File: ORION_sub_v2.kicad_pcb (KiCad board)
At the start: 2 copper layers, 50 x 70 mm, 75 parts, among them J1 Conn_01x02, J10 Conn_01x01, J11 Conn_01x05, J12 Conn_01x03, J13 Conn_01x08, J2 Conn_01x03, J3 Conn_01x04, J4 Conn_01x02, J5 Conn_01x01, J6 Conn_01x04, J7 Conn_01x03, J8 Conn_01x04, J9 Conn_01x01, P1 CONN_01X06, Q1 BSS138, SW1 SW_Push, SW2 SW_Push, SW3 SW_Push, SW4 SW_Push, U1 STM32F303CBTx, U2 MAX3051, U3 AZ1117-3.3, U4 BD9G101G, X1 ceralock

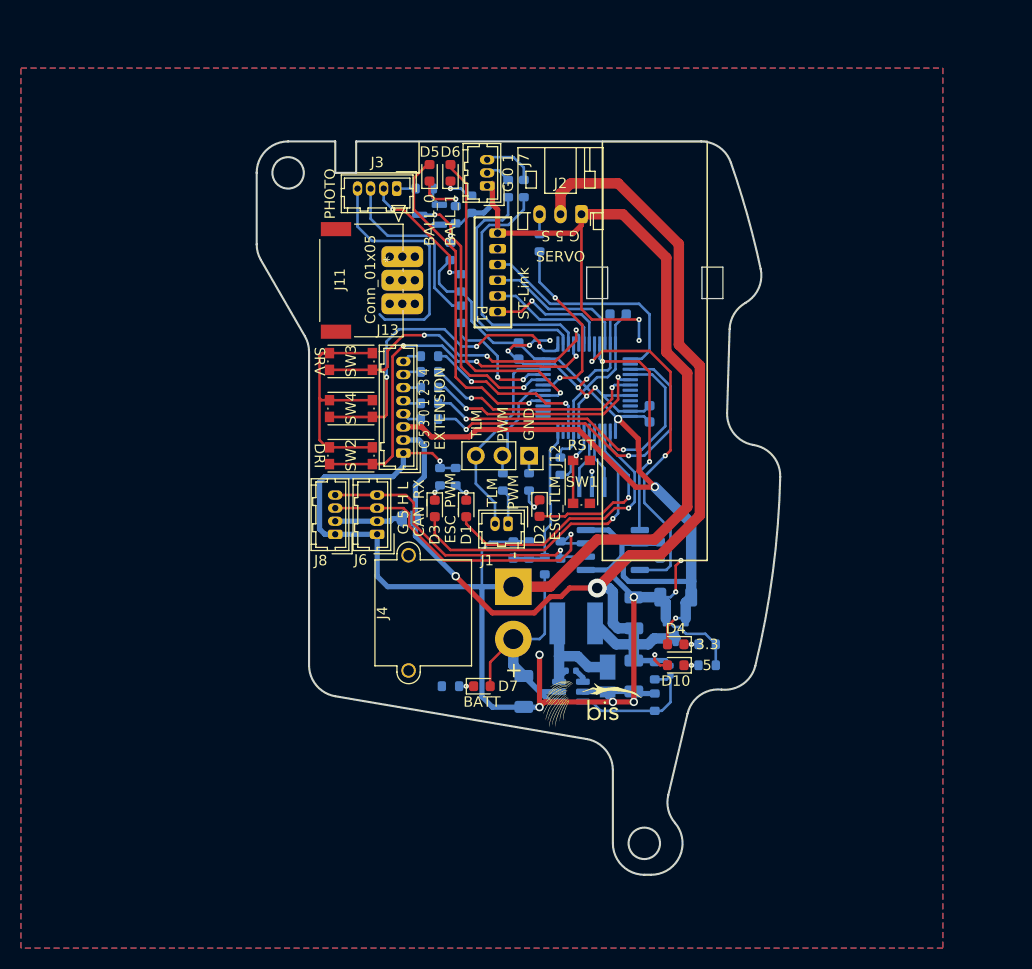
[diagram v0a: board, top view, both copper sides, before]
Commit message: 更新
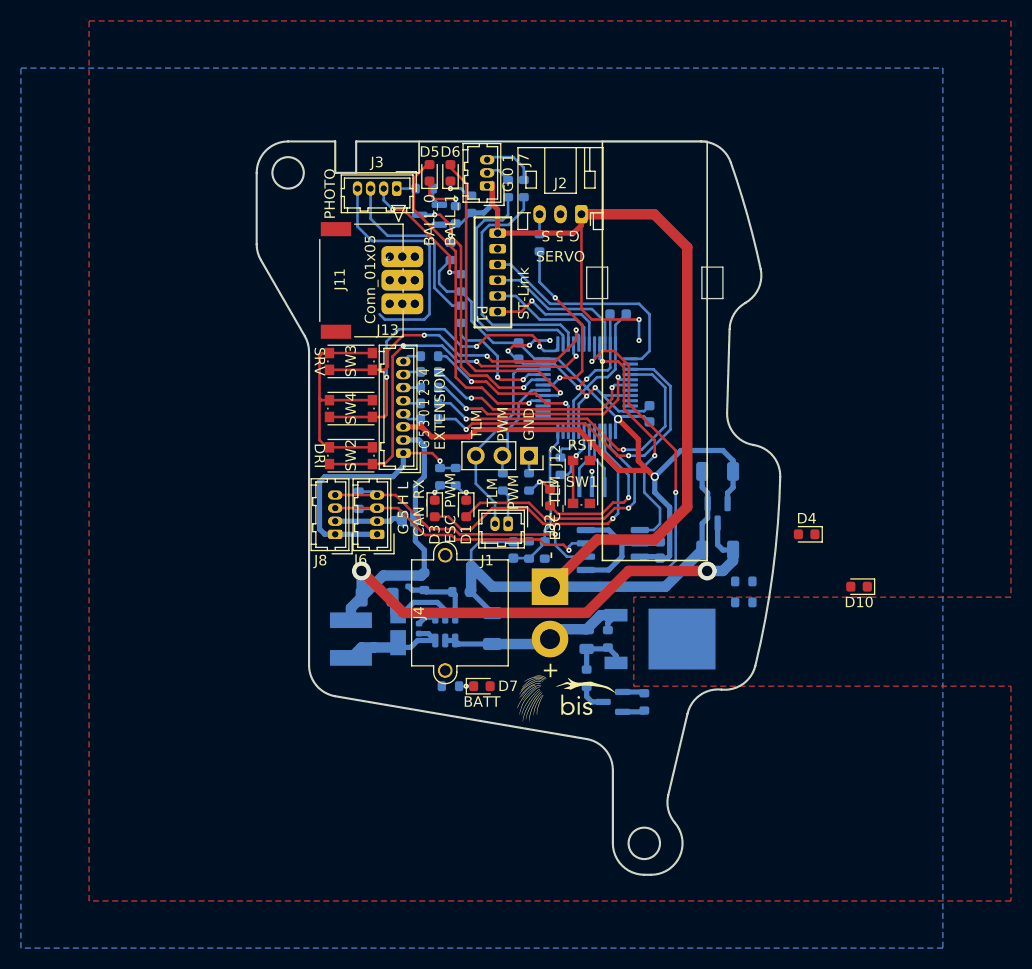
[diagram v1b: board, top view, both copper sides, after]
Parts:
- added D8: D_Zener, Diode_SMD:D_0805_2012Metric, B.Cu at (120.0, 102.0)
- added Q2: Q_PMOS_GDS, Package_TO_SOT_SMD:TO-252-2, B.Cu at (127.0, 102.0)
- added Q3: BSS138, Package_TO_SOT_SMD:SOT-23, B.Cu at (122.5, 108.0)
- added R28: 1k, Resistor_SMD:R_0603_1608Metric, B.Cu at (120.0, 105.7)
- added R29: 1k, Resistor_SMD:R_0603_1608Metric, B.Cu at (122.0, 102.0)
- added R30: 1k, Resistor_SMD:R_0603_1608Metric, B.Cu at (125.5, 108.0)
- moved C4 26.4 mm to (103.0, 96.5)
- moved C13 25.6 mm to (100.0, 98.0), turned to 0 degrees
- moved R16 23.6 mm to (104.5, 96.5)
- moved L1 21.6 mm to (97.5, 102.0), turned to 90 degrees
- moved R15 21.3 mm to (108.0, 97.5), turned to 180 degrees
- moved D9 20.4 mm to (102.0, 101.5), turned to 90 degrees
- moved R2 19.8 mm to (98.2, 88.8), turned to -90 degrees
- moved D10 19.0 mm to (146.0, 97.0)
- moved D4 16.3 mm to (141.0, 92.0)
- moved C3 15.0 mm to (104.0, 101.0), turned to 90 degrees
- moved U4 13.4 mm to (106.5, 101.0), turned to -90 degrees
- moved C8 12.6 mm to (132.5, 86.0)
- moved U3 11.7 mm to (132.5, 90.0)
- moved C7 10.0 mm to (132.5, 93.5), turned to 180 degrees
- moved R17 6.95 mm to (135.0, 98.5)
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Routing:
- net +5V: track 115.4 -> 71.1 mm, vias 3 -> 2
- net GND: track 315.1 -> 272.3 mm, vias 18 -> 11
- net +3.3V: track 112.9 -> 105.5 mm, vias 3 -> 2
- net +BATT: track 26.6 -> 19.3 mm
- net Net-(C4-Pad2): track 13.2 -> 6.87 mm
- net Net-(D8-Pad2): track 0.00 -> 5.86 mm
- net /CAN_RX: track 34.2 -> 30.5 mm
- net /CAN_H: track 30.9 -> 27.9 mm
- net Net-(Q3-Pad3): track 0.00 -> 2.71 mm
- net /ESC_BATT_EN: track 0.00 -> 2.11 mm
- net Net-(C3-Pad1): track 11.6 -> 13.0 mm
- net /LED_2: track 29.8 -> 28.4 mm
- net Net-(D4-Pad1): track 1.39 -> 0.00 mm, vias 1 -> 0
- net Net-(D10-Pad1): track 1.39 -> 0.00 mm, vias 1 -> 0
- net /LED_0: track 27.0 -> 25.6 mm
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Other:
- board text removed: "3.3"
- board text removed: "5"
